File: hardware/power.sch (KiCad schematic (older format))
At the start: 19 parts, among them J4 Barrel_Jack, U18 LT1528CQ, U19 LT1529CQ#PBF

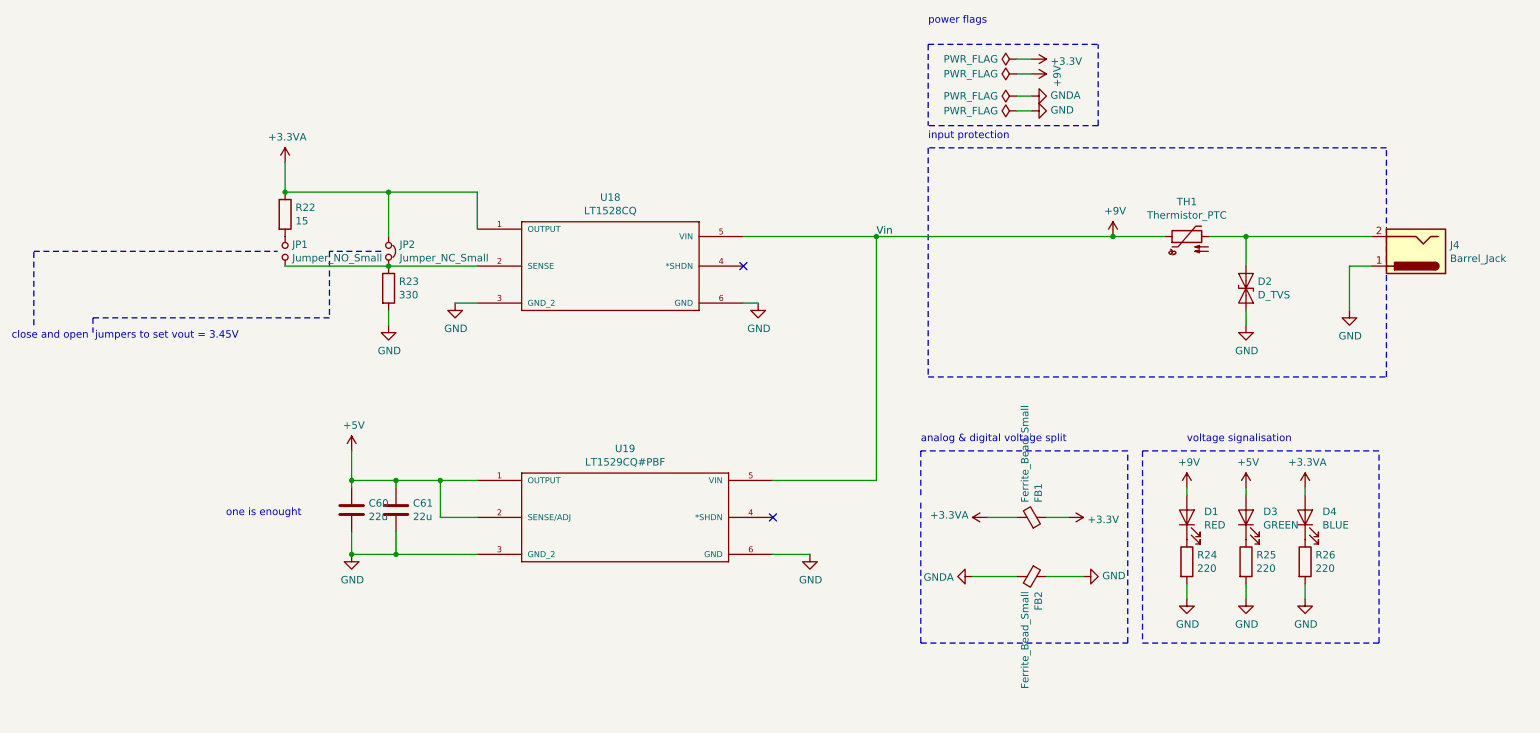
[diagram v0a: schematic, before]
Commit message: pierwszy układ PCB
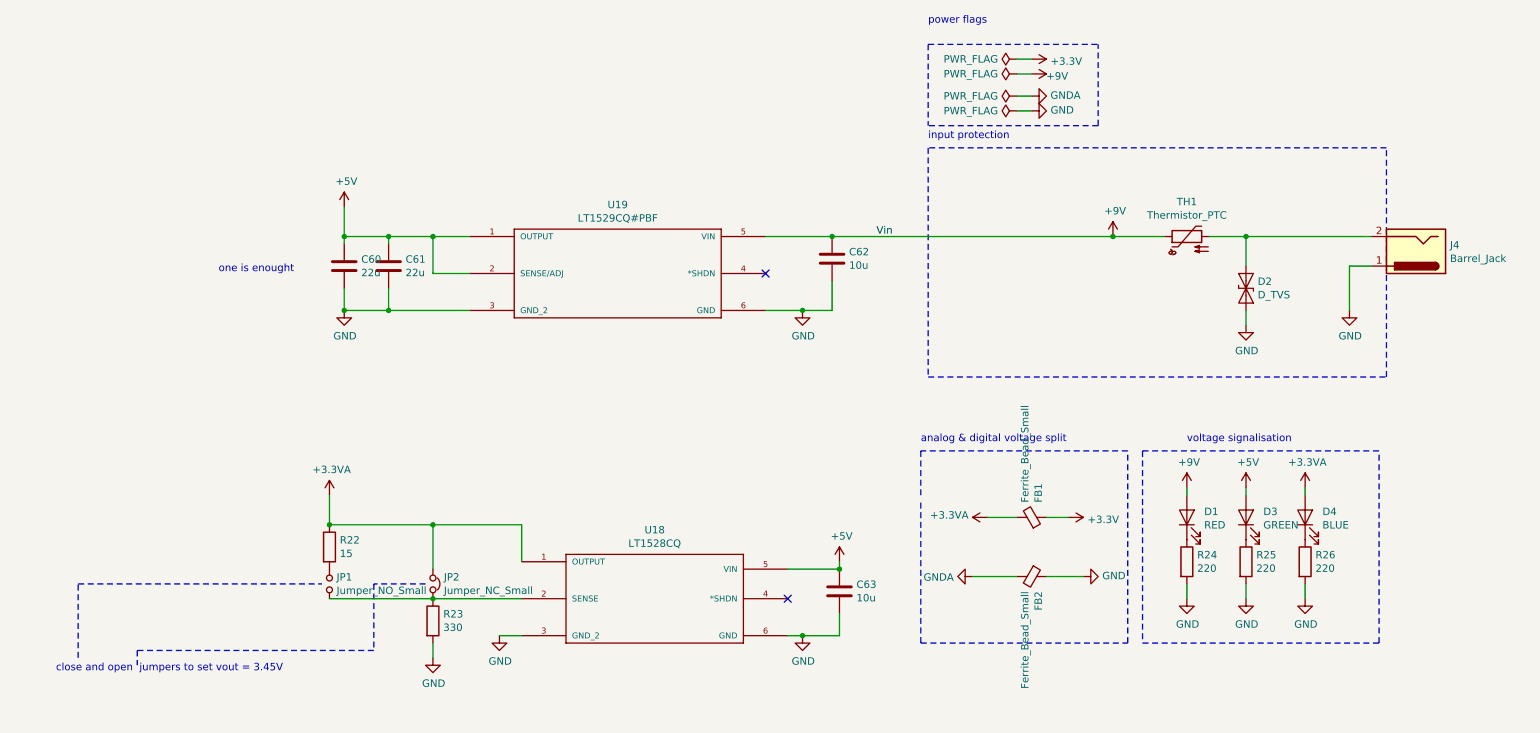
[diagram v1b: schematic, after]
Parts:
- added C62, C63: 10u, Capacitor_SMD:C_0805_2012Metric_Pad1.15x1.40mm_HandSolder, symbol Device:C
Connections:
- net +5V: now also U18.5 (VIN), C63.1
- net +9V: now also C62.1; no longer U18.5 (VIN)
- net GND: now also C62.2, C63.2
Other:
- moved on the sheet: C60, C61, JP1, JP2, R22, R23, U18, U19
